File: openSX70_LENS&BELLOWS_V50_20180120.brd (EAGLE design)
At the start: 95.9 x 27.9 mm, 47 parts, among them Q1 5.8A/30V/35mΩ, Q2 5.8A/30V/35mΩ, U1 ATMEGA328P_TQFP, U3 BH1750FVI-TR, Y1 CSTCE16M0V53-R0

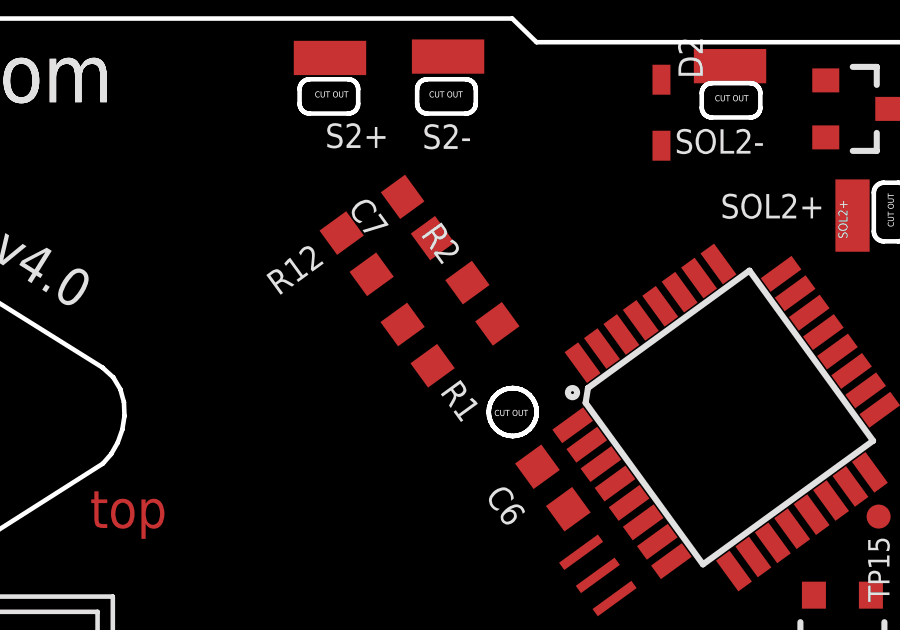
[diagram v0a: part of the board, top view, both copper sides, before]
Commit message: Lost track of what I was doing, but basically trying to stay out of the light seal.
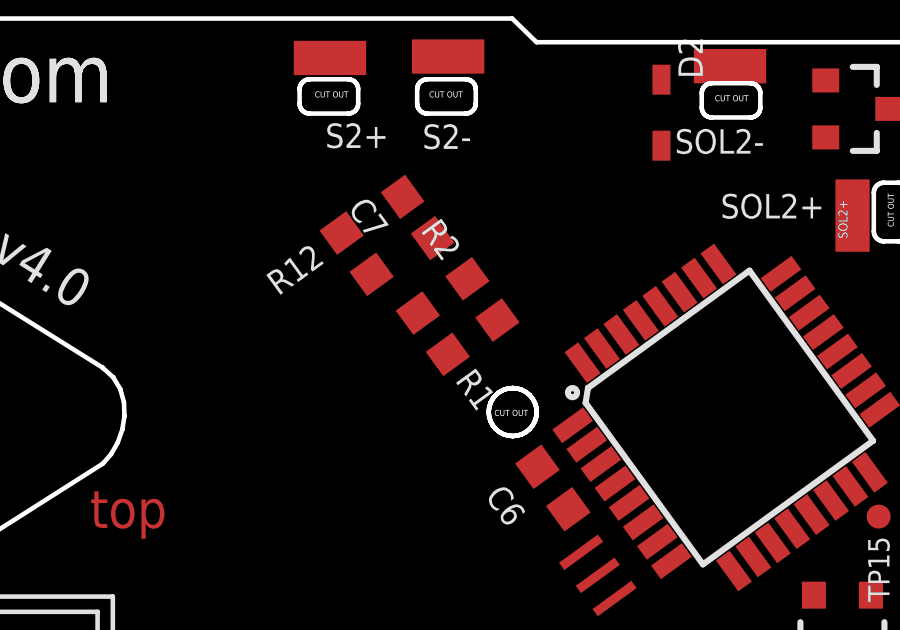
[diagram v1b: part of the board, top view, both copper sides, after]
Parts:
- moved R1 0.64 mm to (71.1, 18.2)
- moved R2 0.13 mm to (72.8, 19.3)
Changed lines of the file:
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@@
 <attribute name="VALUE" x="85.217" y="24.003" size="0.6096" layer="27" font="vector" ratio="20" align="top-center"/>
 </element>
-<element name="R1" library="resistor" library_urn="urn:adsk.eagle:library:348" package="R0603" package3d_urn="urn:adsk.eagle:package:26057/1" value="100R" x="70.612" y="17.78" smashed="yes" rot="R126">
-<attribute name="NAME" x="72.7702" y="15.619734375" size="0.8128" layer="25" font="vector" ratio="20" rot="R126"/>
-<attribute name="VALUE" x="69.75395" y="19.8252625" size="0.8128" layer="27" font="vector" rot="R126"/>
+<element name="R1" library="resistor" library_urn="urn:adsk.eagle:library:348" package="R0603" package3d_urn="urn:adsk.eagle:package:26057/1" value="100R" x="71.12" y="18.161" smashed="yes" rot="R126">
+<attribute name="NAME" x="73.2782" y="16.000734375" size="0.8128" layer="25" font="vector" ratio="20" rot="R126"/>
+<attribute name="VALUE" x="70.26195" y="20.2062625" size="0.8128" layer="27" font="vector" rot="R126"/>
 </element>
 <element name="R10" library="resistor" library_urn="urn:adsk.eagle:library:348" package="R0603" package3d_urn="urn:adsk.eagle:package:26057/1" value="15K" x="26.3525" y="21.717" smashed="yes" rot="R180">
@@
 <attribute name="VALUE" x="15.875" y="20.47875" size="1.27" layer="28" rot="MR0"/>
 </element>
-<element name="R2" library="resistor" library_urn="urn:adsk.eagle:library:348" package="R0603" package3d_urn="urn:adsk.eagle:package:26057/1" value="100K" x="72.771" y="19.177" smashed="yes" rot="R126">
-<attribute name="NAME" x="72.129871875" y="20.869678125" size="0.8128" layer="25" font="vector" ratio="20" rot="R126"/>
-<attribute name="VALUE" x="75.46799375" y="16.1131" size="0.8128" layer="27" font="vector" rot="R126"/>
+<element name="R2" library="resistor" library_urn="urn:adsk.eagle:library:348" package="R0603" package3d_urn="urn:adsk.eagle:package:26057/1" value="100K" x="72.771" y="19.304" smashed="yes" rot="R126">
+<attribute name="NAME" x="72.129871875" y="20.996678125" size="0.8128" layer="25" font="vector" ratio="20" rot="R126"/>
+<attribute name="VALUE" x="75.46799375" y="16.2401" size="0.8128" layer="27" font="vector" rot="R126"/>
 </element>
 <element name="R3" library="resistor" library_urn="urn:adsk.eagle:library:348" package="R0603" package3d_urn="urn:adsk.eagle:package:26057/1" value="100R" x="90.6145" y="25.527" smashed="yes" rot="R90">
@@
 <contactref element="R1" pad="1"/>
 <contactref element="U1" pad="1"/>
-<wire x1="71.111615625" y1="17.092334375" x2="75.7804125" y2="15.10911875" width="0" layer="19" extent="1-1"/>
+<wire x1="71.619615625" y1="17.473334375" x2="75.7804125" y2="15.10911875" width="0" layer="19" extent="1-1"/>
 </signal>
 <signal name="BUZZER">
@@
 <wire x1="84.217" y1="24.704" x2="84.136671875" y2="18.21373125" width="0" layer="19" extent="1-1"/>
 <wire x1="88.392" y1="24.677" x2="84.217" y2="24.704" width="0" layer="19" extent="1-1"/>
-<wire x1="73.270615625" y1="18.489334375" x2="88.392" y2="24.677" width="0" layer="19" extent="1-1"/>
-<wire x1="76.72086875" y1="13.814690625" x2="73.270615625" y2="18.489334375" width="0" layer="19" extent="1-1"/>
+<wire x1="73.270615625" y1="18.616334375" x2="88.392" y2="24.677" width="0" layer="19" extent="1-1"/>
+<wire x1="76.72086875" y1="13.814690625" x2="73.270615625" y2="18.616334375" width="0" layer="19" extent="1-1"/>
 <wire x1="77.661325" y1="12.520265625" x2="76.72086875" y2="13.814690625" width="0" layer="19" extent="1-1"/>
 <wire x1="74.6061875" y1="13.7253875" x2="76.72086875" y2="13.814690625" width="0" layer="19" extent="1-1"/>
@@
 <contactref element="Q1" pad="1"/>
 <contactref element="R2" pad="2"/>
-<wire x1="70.11238125" y1="18.4676625" x2="72.27138125" y2="19.8646625" width="0" layer="19" extent="1-1"/>
-<wire x1="85.7225" y1="9.4455" x2="72.27138125" y2="19.8646625" width="0" layer="19" extent="1-1"/>
+<wire x1="70.62038125" y1="18.8486625" x2="72.27138125" y2="19.9916625" width="0" layer="19" extent="1-1"/>
+<wire x1="85.7225" y1="9.4455" x2="72.27138125" y2="19.9916625" width="0" layer="19" extent="1-1"/>
 </signal>
 <signal name="N$3">
